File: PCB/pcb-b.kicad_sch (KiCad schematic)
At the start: 23 parts, among them Q13 TPCA8120,L1Q, Q9 BC817, U1 L7805, U2 L7805, U3 L7805

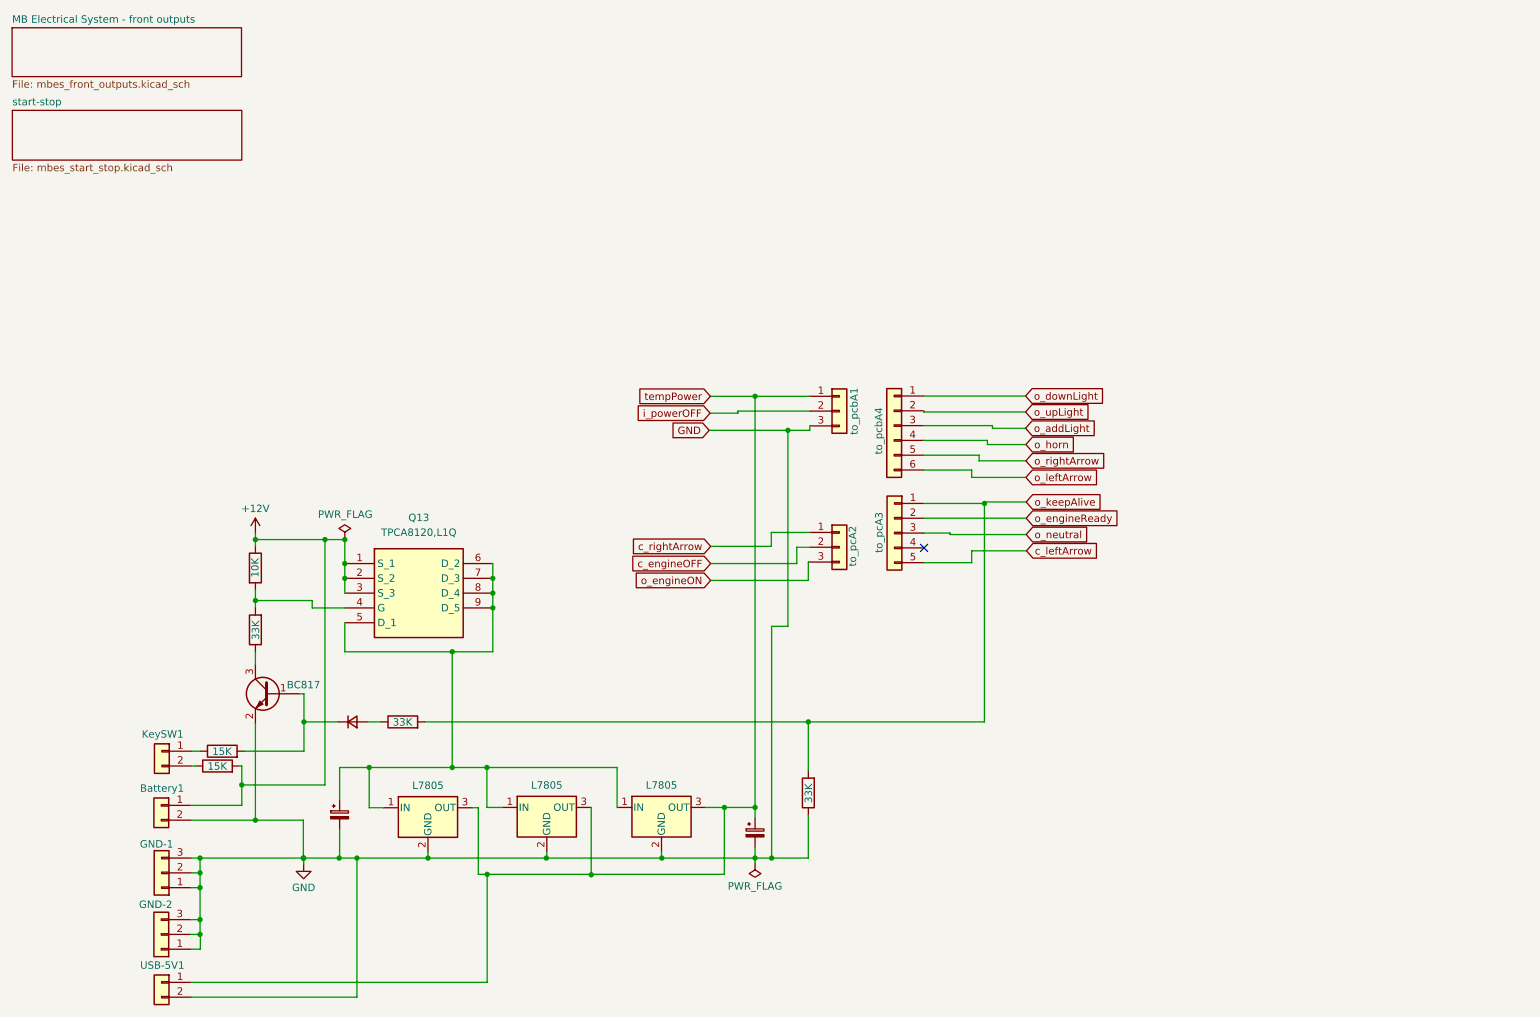
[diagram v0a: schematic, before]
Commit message: Manual merging from the ATmega16__dualPCB branch
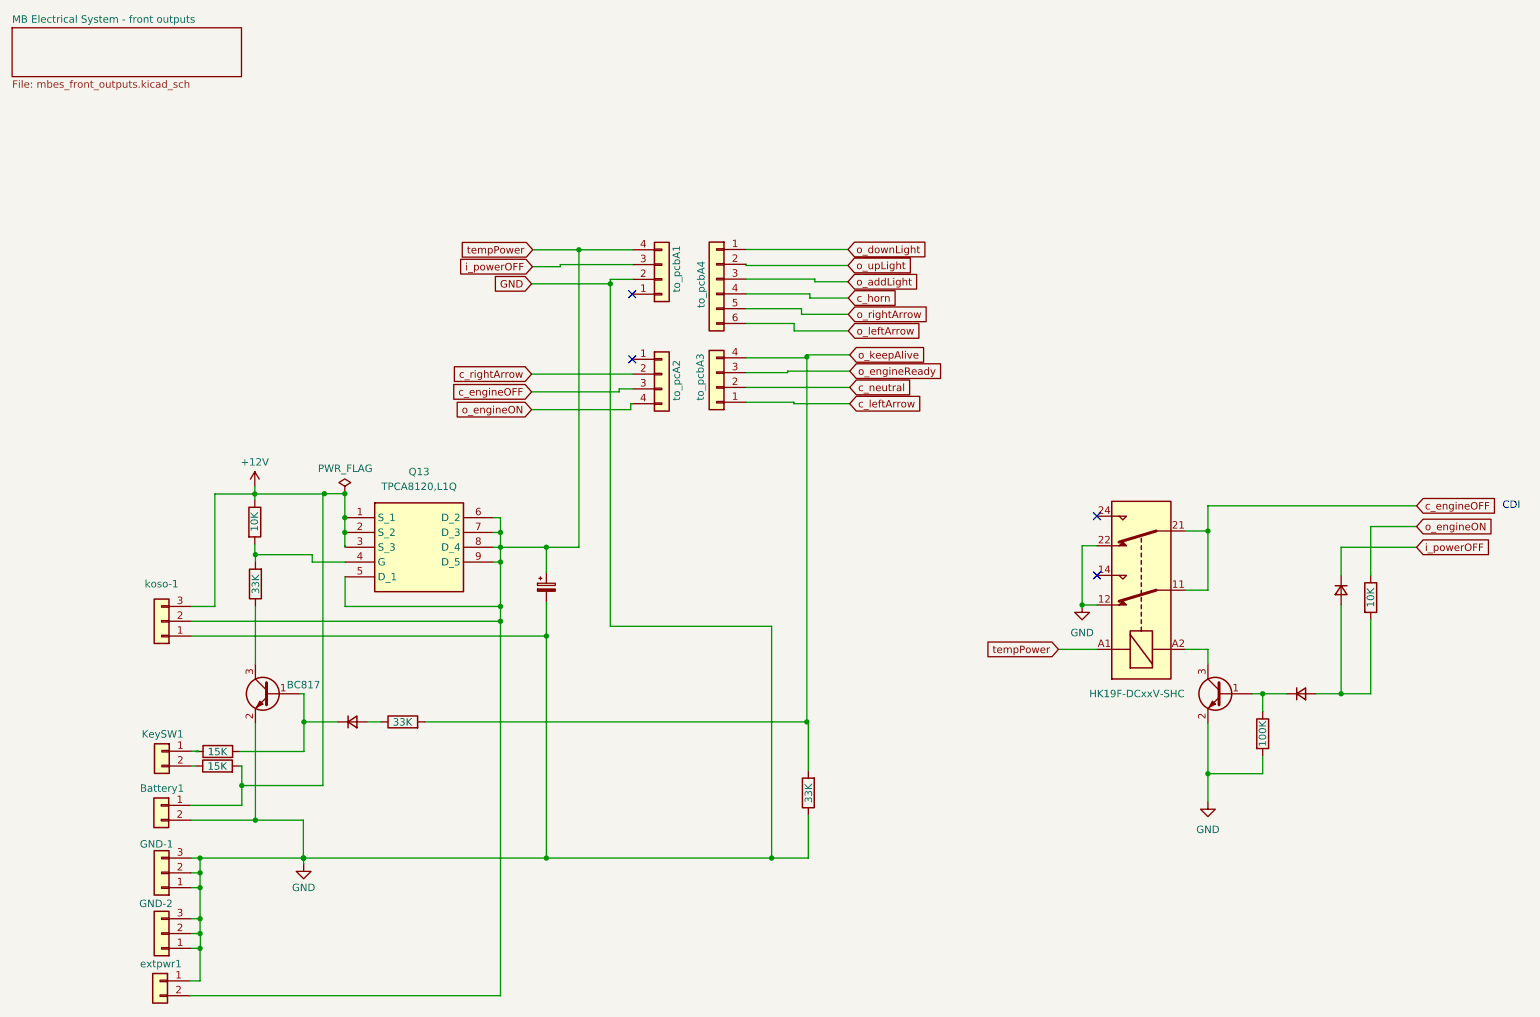
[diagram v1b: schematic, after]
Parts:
- removed C1: C_Polarized_Small, Capacitor_THT:CP_Radial_D8.0mm_P2.50mm, symbol Device:C_Polarized_Small
- removed U1, U2, U3: L7805, Package_TO_SOT_THT:TO-220-3_Vertical, symbol Regulator_Linear:L7805
- removed USB-5V1: Conn_01x02, Connector_Wire:SolderWire-0.75sqmm_1x02_P7mm_D1.25mm_OD3.5mm, symbol Connector_Generic:Conn_01x02
- removed to_pcA2, to_pcbA1: Conn_01x03, Connector_PinSocket_2.54mm:PinSocket_1x03_P2.54mm_Vertical, symbol Connector_Generic:Conn_01x03
- removed to_pcA3: Conn_01x05, Connector_PinSocket_2.54mm:PinSocket_1x05_P2.54mm_Vertical, symbol Connector_Generic:Conn_01x05
- added D2, D3: D_Small, Diode_SMD:D_1210_3225Metric_Pad1.42x2.65mm_HandSolder, symbol Device:D_Small
- added K1: HK19F-DCxxV-SHC, Relay_THT:Relay_DPDT_Finder_30.22, symbol Relay:HK19F-DCxxV-SHC
- added Q3: BC817, Package_TO_SOT_SMD:SOT-23, symbol Transistor_BJT:BC817
- added RA15: 10K, Resistor_SMD:R_1206_3216Metric, symbol Device:R
- added RA8: 100K, Resistor_SMD:R_1206_3216Metric, symbol Device:R
- added extpwr1: Conn_01x02, Connector_PinHeader_2.54mm:PinHeader_1x02_P2.54mm_Vertical, symbol Connector_Generic:Conn_01x02
- added koso-1: Conn_01x03, Connector_PinHeader_2.54mm:PinHeader_1x03_P2.54mm_Vertical, symbol Connector_Generic:Conn_01x03
- added to_pcA2, to_pcbA1, to_pcbA3: Conn_01x04, Connector_PinSocket_2.54mm:PinSocket_1x04_P2.54mm_Vertical, symbol Connector_Generic:Conn_01x04
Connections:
- net +12V: now also koso-1.3 (Pin_3)
- net GND: now also K1.12, K1.22, Q3.2 (E), RA8.2, extpwr1.1 (Pin_1), koso-1.1 (Pin_1), to_pcbA1.2 (Pin_2)
- net c_engineOFF: now also K1.11, K1.21, to_pcA2.3 (Pin_3)
- net c_leftArrow: now also to_pcbA3.1 (Pin_1)
- net c_rightArrow: now also to_pcA2.2 (Pin_2)
- net i_powerOFF: now also D3.1 (K), to_pcbA1.3 (Pin_3)
- net o_engineON: now also RA15.1, to_pcA2.4 (Pin_4)
- net o_engineReady: now also to_pcbA3.3 (Pin_3)
- net o_keepAlive: now also to_pcbA3.4 (Pin_4)
- net tempPower: now also C9.1, Q13.5 (D_1), Q13.6 (D_2), Q13.7 (D_3), Q13.8 (D_4), Q13.9 (D_5), K1.A1, extpwr1.2 (Pin_2), koso-1.2 (Pin_2), to_pcbA1.4 (Pin_4)
- net o_horn renamed c_horn
- new net: D2.1 (K), Q3.1 (B), RA8.1
- new net: K1.A2, Q3.3 (C)
- new net: D2.2 (A), D3.2 (A), RA15.2
- new net c_neutral: to_pcbA3.2 (Pin_2)
- no-connect marks 1 -> 4
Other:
- removed sheet start-stop
- note added: "CDI"
- moved on the sheet: Q13, to_pcbA4

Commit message: Old files replaced.
They have been merged for error
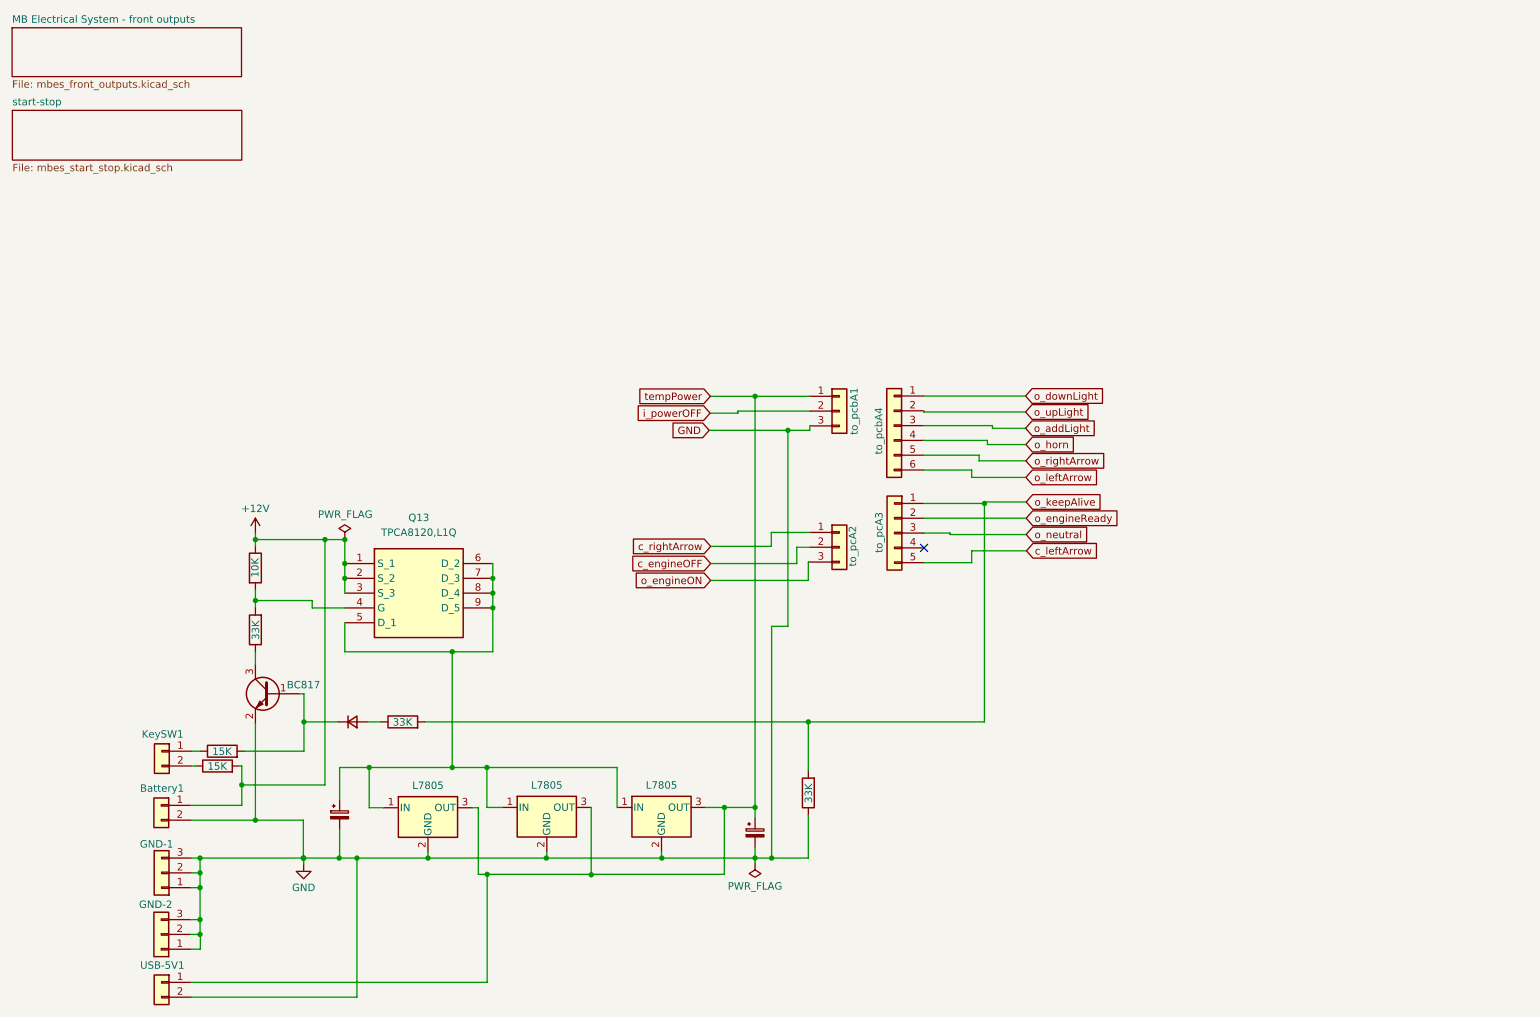
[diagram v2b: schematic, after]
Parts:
- removed D2, D3: D_Small, Diode_SMD:D_1210_3225Metric_Pad1.42x2.65mm_HandSolder, symbol Device:D_Small
- removed K1: HK19F-DCxxV-SHC, Relay_THT:Relay_DPDT_Finder_30.22, symbol Relay:HK19F-DCxxV-SHC
- removed Q3: BC817, Package_TO_SOT_SMD:SOT-23, symbol Transistor_BJT:BC817
- removed RA15: 10K, Resistor_SMD:R_1206_3216Metric, symbol Device:R
- removed RA8: 100K, Resistor_SMD:R_1206_3216Metric, symbol Device:R
- removed extpwr1: Conn_01x02, Connector_PinHeader_2.54mm:PinHeader_1x02_P2.54mm_Vertical, symbol Connector_Generic:Conn_01x02
- removed koso-1: Conn_01x03, Connector_PinHeader_2.54mm:PinHeader_1x03_P2.54mm_Vertical, symbol Connector_Generic:Conn_01x03
- removed to_pcA2, to_pcbA1, to_pcbA3: Conn_01x04, Connector_PinSocket_2.54mm:PinSocket_1x04_P2.54mm_Vertical, symbol Connector_Generic:Conn_01x04
- added C1: C_Polarized_Small, Capacitor_THT:CP_Radial_D8.0mm_P2.50mm, symbol Device:C_Polarized_Small
- added U1, U2, U3: L7805, Package_TO_SOT_THT:TO-220-3_Vertical, symbol Regulator_Linear:L7805
- added USB-5V1: Conn_01x02, Connector_Wire:SolderWire-0.75sqmm_1x02_P7mm_D1.25mm_OD3.5mm, symbol Connector_Generic:Conn_01x02
- added to_pcA2, to_pcbA1: Conn_01x03, Connector_PinSocket_2.54mm:PinSocket_1x03_P2.54mm_Vertical, symbol Connector_Generic:Conn_01x03
- added to_pcA3: Conn_01x05, Connector_PinSocket_2.54mm:PinSocket_1x05_P2.54mm_Vertical, symbol Connector_Generic:Conn_01x05
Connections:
- net GND: now also C1.2, U1.2 (GND), U2.2 (GND), U3.2 (GND), USB-5V1.2 (Pin_2), to_pcbA1.3 (Pin_3)
- net c_engineOFF: now also to_pcA2.2 (Pin_2)
- net c_leftArrow: now also to_pcA3.5 (Pin_5)
- net c_rightArrow: now also to_pcA2.1 (Pin_1)
- net i_powerOFF: now also to_pcbA1.2 (Pin_2)
- net o_engineON: now also to_pcA2.3 (Pin_3)
- net o_engineReady: now also to_pcA3.2 (Pin_2)
- net o_keepAlive: now also to_pcA3.1 (Pin_1)
- net tempPower: now also C1.1, U1.3 (OUT), U2.3 (OUT), U3.3 (OUT), USB-5V1.1 (Pin_1), to_pcbA1.1 (Pin_1); no longer C9.1, Q13.5 (D_1), Q13.6 (D_2), Q13.7 (D_3), Q13.8 (D_4), Q13.9 (D_5)
- net c_horn renamed o_horn
- new net: C9.1, Q13.5 (D_1), Q13.6 (D_2), Q13.7 (D_3), Q13.8 (D_4), Q13.9 (D_5), U1.1 (IN), U2.1 (IN), U3.1 (IN)
- new net o_neutral: to_pcA3.3 (Pin_3)
- no-connect marks 4 -> 1
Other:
- added sheet start-stop (mbes_start_stop.kicad_sch)
- note removed: "CDI"
- moved on the sheet: Q13, to_pcbA4
